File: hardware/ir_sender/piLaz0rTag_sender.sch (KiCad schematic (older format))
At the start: 2 parts

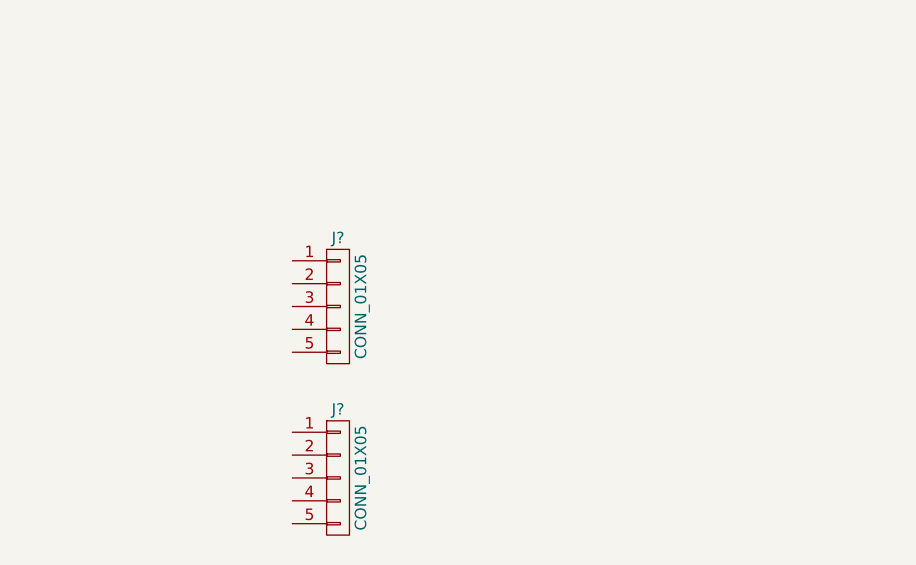
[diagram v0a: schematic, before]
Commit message: Add ir sender gerber files
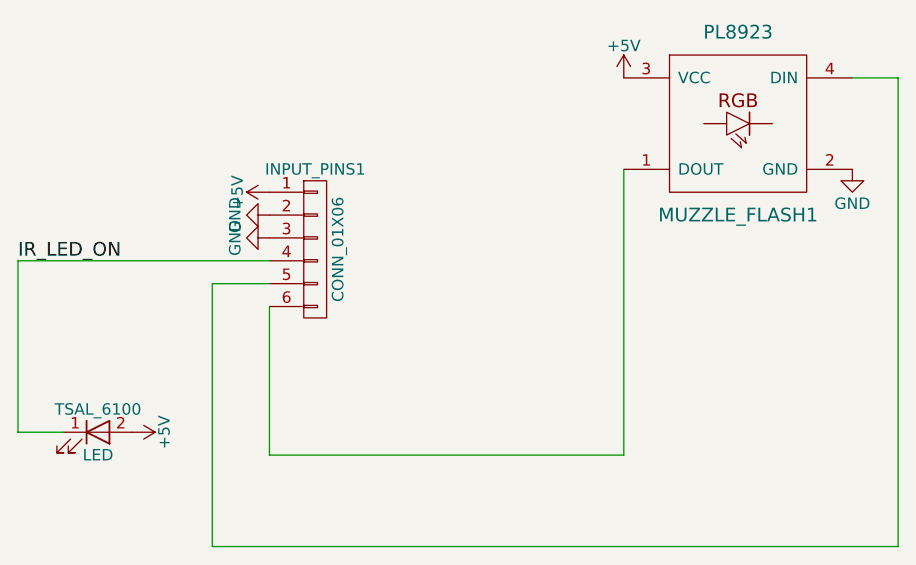
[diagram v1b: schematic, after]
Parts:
- removed J? (x2): CONN_01X05, symbol CONN_01X05
- added INPUT_PINS1: CONN_01X06, Socket_Strips:Socket_Strip_Straight_1x06_Pitch2.54mm, symbol CONN_01X06
- added MUZZLE_FLASH1: PL8923, Socket_Strips:Socket_Strip_Straight_1x04_Pitch2.54mm, symbol PL8923
- added TSAL_6100: LED, LEDs:LED_D5.0mm, symbol LED
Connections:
- new net: INPUT_PINS1.6 (P6), MUZZLE_FLASH1.1 (DOUT)
- new net: INPUT_PINS1.5 (P5), MUZZLE_FLASH1.4 (DIN)
- new net +5V: INPUT_PINS1.1 (P1), MUZZLE_FLASH1.3 (VCC), TSAL_6100.2 (A)
- new net GND: INPUT_PINS1.2 (P2), INPUT_PINS1.3 (P3), MUZZLE_FLASH1.2 (GND)
- new net IR_LED_ON: INPUT_PINS1.4 (P4), TSAL_6100.1 (K)
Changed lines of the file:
@@
 LIBS:atmel
 LIBS:contrib
+LIBS:pl8923
 LIBS:valves
-LIBS:shardy
+LIBS:piLaz0rTag_sender-cache
 EELAYER 25 0
 EELAYER END
@@
 $EndDescr
 $Comp
-L CONN_01X05 J?
-U 1 1 58F64742
-P 3050 2800
-F 0 "J?" H 3050 3100 50  0000 C CNN
-F 1 "CONN_01X05" V 3150 2800 50  0000 C CNN
-F 2 "" H 3050 2800 50  0001 C CNN
-F 3 "" H 3050 2800 50  0001 C CNN
-	1    3050 2800
+L LED TSAL_6100
+U 1 1 590CAF89
+P 2000 2600
+F 0 "TSAL_6100" H 2000 2700 50  0000 C CNN
+F 1 "LED" H 2000 2500 50  0000 C CNN
+F 2 "LEDs:LED_D5.0mm" H 2000 2600 50  0001 C CNN
+F 3 "" H 2000 2600 50  0001 C CNN
+	1    2000 2600
 	1    0    0    -1
 $EndComp
 $Comp
-L CONN_01X05 J?
-U 1 1 58F6478D
-P 3050 2050
-F 0 "J?" H 3050 2350 50  0000 C CNN
-F 1 "CONN_01X05" V 3150 2050 50  0000 C CNN
-F 2 "" H 3050 2050 50  0001 C CNN
-F 3 "" H 3050 2050 50  0001 C CNN
-	1    3050 2050
+L +5V #PWR1
+U 1 1 590CB056
+P 2150 2600
+F 0 "#PWR1" H 2150 2450 50  0001 C CNN
+F 1 "+5V" H 2150 2740 50  0000 C CNN
+F 2 "" H 2150 2600 50  0001 C CNN
+F 3 "" H 2150 2600 50  0001 C CNN
+	1    2150 2600
+	0    1    1    0
+$EndComp
+$Comp
+L PL8923 MUZZLE_FLASH1
+U 1 1 590CB0E6
+P 4800 1250
+F 0 "MUZZLE_FLASH1" H 4800 850 60  0000 C CNN
+F 1 "PL8923" H 4800 1650 60  0000 C CNN
+F 2 "Socket_Strips:Socket_Strip_Straight_1x04_Pitch2.54mm" V 4750 1250 60  0001 C CNN
+F 3 "" V 4750 1250 60  0000 C CNN
+	1    4800 1250
 	1    0    0    -1
 $EndComp
+$Comp
+L GND #PWR5
+U 1 1 590CB177
+P 5300 1450
+F 0 "#PWR5" H 5300 1200 50  0001 C CNN
+F 1 "GND" H 5300 1300 50  0000 C CNN
+F 2 "" H 5300 1450 50  0001 C CNN
+F 3 "" H 5300 1450 50  0001 C CNN
+	1    5300 1450
+	1    0    0    -1
+$EndComp
+$Comp
+L +5V #PWR4
+U 1 1 590CB191
+P 4300 1050
+F 0 "#PWR4" H 4300 900 50  0001 C CNN
+F 1 "+5V" H 4300 1190 50  0000 C CNN
+F 2 "" H 4300 1050 50  0001 C CNN
+F 3 "" H 4300 1050 50  0001 C CNN
+	1    4300 1050
+	1    0    0    -1
+$EndComp
+$Comp
+L CONN_01X06 INPUT_PINS1
+U 1 1 590CB4F5
+P 2950 1800
+F 0 "INPUT_PINS1" H 2950 2150 50  0000 C CNN
+F 1 "CONN_01X06" V 3050 1800 50  0000 C CNN
+F 2 "Socket_Strips:Socket_Strip_Straight_1x06_Pitch2.54mm" H 2950 1800 50  0001 C CNN
+F 3 "" H 2950 1800 50  0001 C CNN
+	1    2950 1800
+	1    0    0    -1
+$EndComp
+$Comp
+L +5V #PWR2
+U 1 1 590CB53B
+P 2750 1550
+F 0 "#PWR2" H 2750 1400 50  0001 C CNN
+F 1 "+5V" H 2750 1690 50  0000 C CNN
+F 2 "" H 2750 1550 50  0001 C CNN
+F 3 "" H 2750 1550 50  0001 C CNN
+	1    2750 1550
+	0    -1   -1   0
+$EndComp
+$Comp
+L GND #PWR3
+U 1 1 590CB583
+P 2750 1750
+F 0 "#PWR3" H 2750 1500 50  0001 C CNN
+F 1 "GND" H 2750 1600 50  0000 C CNN
+F 2 "" H 2750 1750 50  0001 C CNN
+F 3 "" H 2750 1750 50  0001 C CNN
+	1    2750 1750
+	0    1    1    0
+$EndComp
+Wire Wire Line
+	2750 1850 1650 1850
+Wire Wire Line
+	1650 1850 1650 2600
+Wire Wire Line
+	1650 2600 1850 2600
+Text Label 1650 1850 0    60   ~ 0
+IR_LED_ON
+Wire Wire Line
+	2750 1950 2500 1950
+Wire Wire Line
+	2500 1950 2500 3100
+Wire Wire Line
+	2500 3100 5500 3100
+Wire Wire Line
+	5500 3100 5500 1050
+Wire Wire Line
+	5500 1050 5300 1050
+Wire Wire Line
+	4300 1450 4300 2700
+Wire Wire Line
+	4300 2700 2750 2700
+Wire Wire Line
+	2750 2700 2750 2050
+$Comp
+L GND #PWR?
+U 1 1 590D8E57
+P 2750 1650
+F 0 "#PWR?" H 2750 1400 50  0001 C CNN
+F 1 "GND" H 2750 1500 50  0000 C CNN
+F 2 "" H 2750 1650 50  0001 C CNN
+F 3 "" H 2750 1650 50  0001 C CNN
+	1    2750 1650
+	0    1    1    0
+$EndComp
 $EndSCHEMATC
